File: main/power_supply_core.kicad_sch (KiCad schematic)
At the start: 47 parts, among them Q201 TK4R3E06PL, Q202 TK4R3E06PL, U101 ZXCT1110, U202 TPS43060

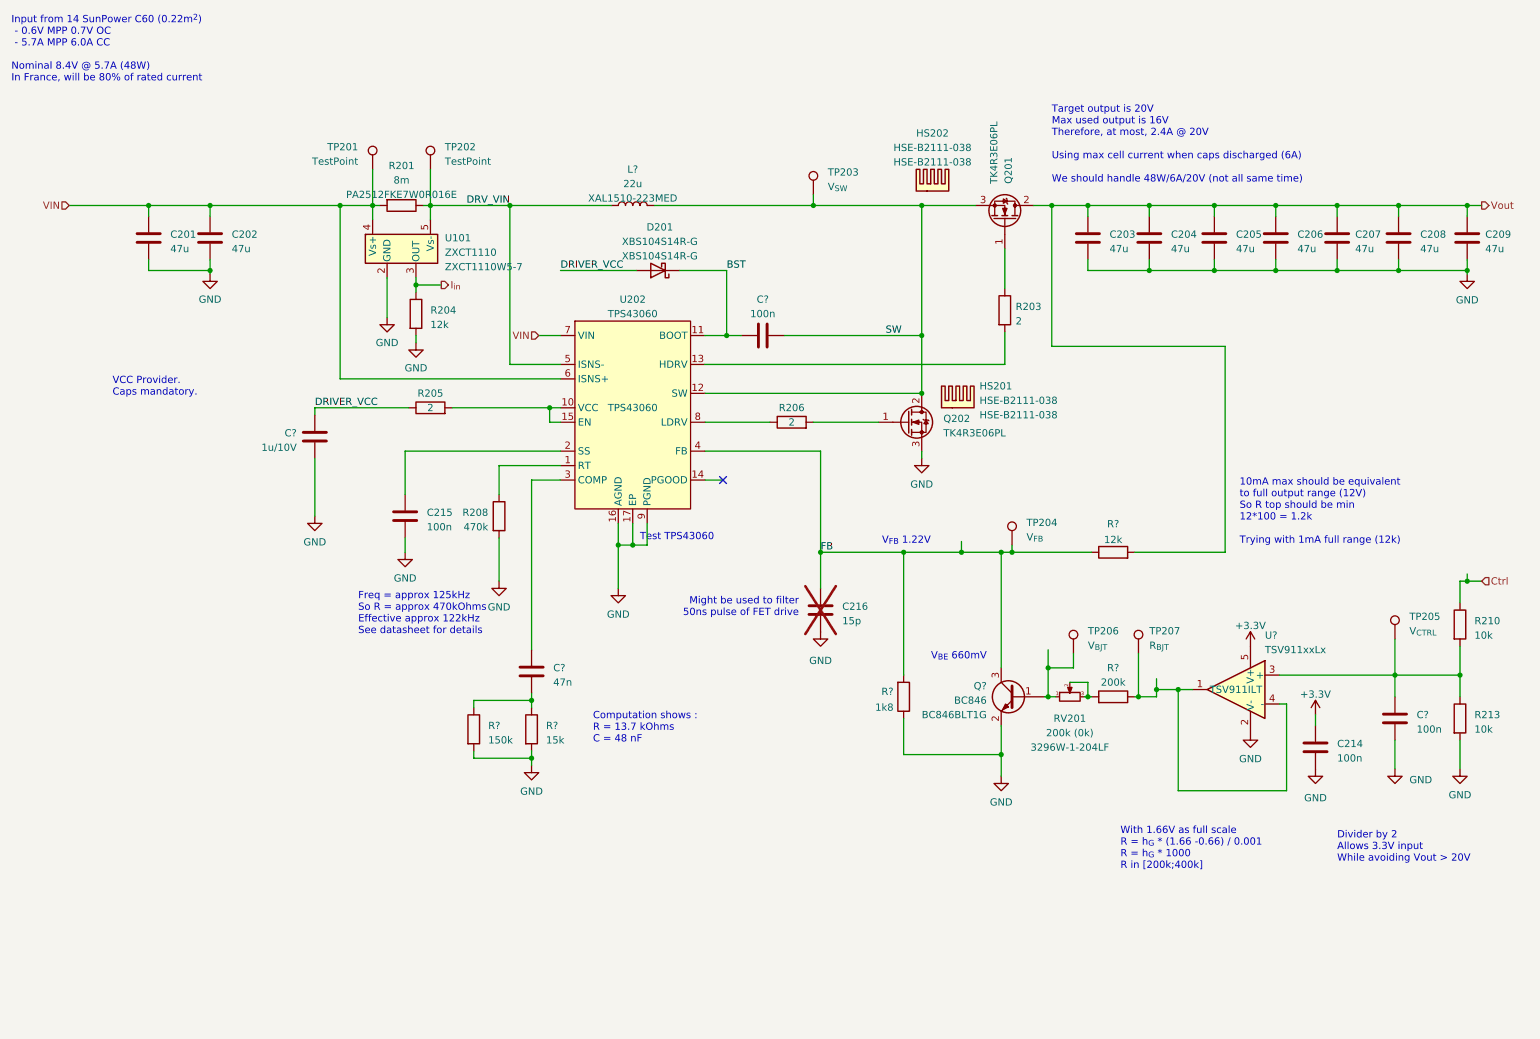
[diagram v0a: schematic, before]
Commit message: Start overall new board
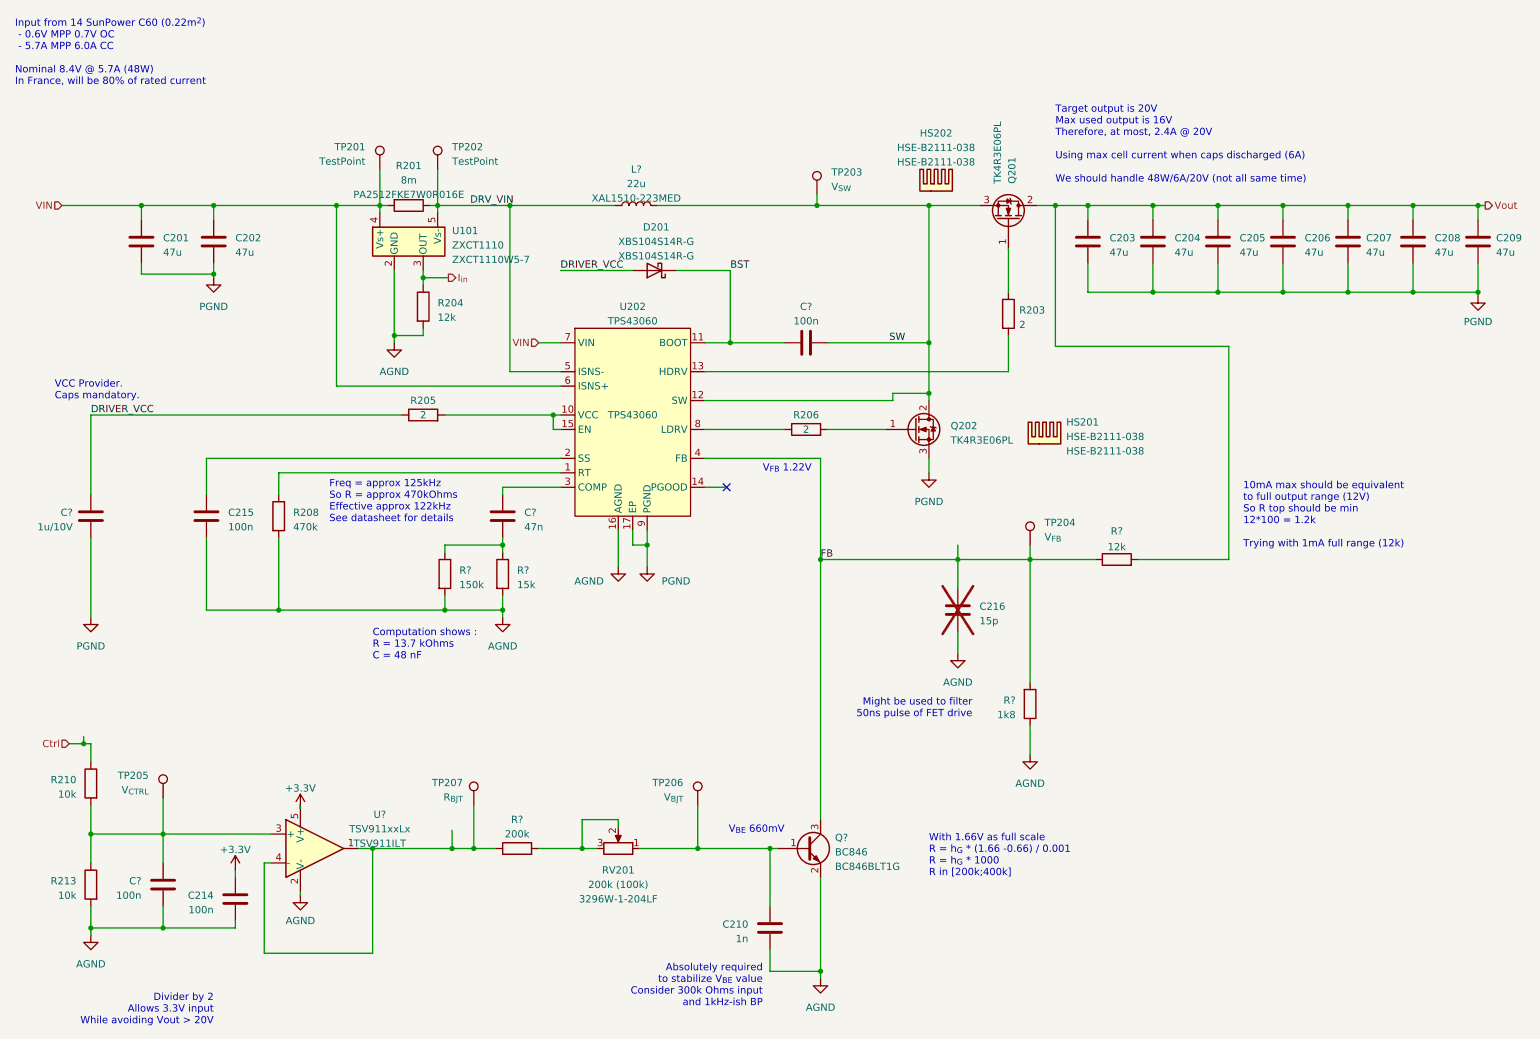
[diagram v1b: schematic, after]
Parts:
- added C210: 1n, Capacitor_SMD:C_0805_2012Metric, symbol Device:C
- RV201: value 200k (0k) -> 200k (100k); symbol Device:R_Potentiometer_Small -> Device:R_Potentiometer
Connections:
- net at Q?.1 (B), RV201.1, TP206.1: now also C210.1
- net GND renamed AGND
- net AGND: now also C210.2; no longer C201.2, C202.2, C203.2, C204.2, C205.2, C206.2, C207.2, C208.2, C209.2, C?.2, Q202.3 (S), U202.17 (EP), U202.9 (PGND)
- new net PGND: C201.2, C202.2, C203.2, C204.2, C205.2, C206.2, C207.2, C208.2, C209.2, C?.2, Q202.3 (S), U202.17 (EP), U202.9 (PGND)
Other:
- note added: "Absolutely required to stabilize V_{BE} value Consider 300k Ohms input and 1kHz-ish BP"
- note removed: "Test TPS43060"
- moved on the sheet: C201, C202, C203, C204, C205, C206, C207, C208, C209, C214, C215, C216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

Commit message: Start design of new PSU
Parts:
- L?, Q?: Spice_Netlist_Enabled Y -> (none)
- U?: Spice_Netlist_Enabled N -> (none)
